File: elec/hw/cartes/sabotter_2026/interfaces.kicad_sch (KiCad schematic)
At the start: 49 parts, among them J10 2-1445051-3, J11 22272051, J12 22272031, J13 3-794630-6, J6 3-794630-4, J9 3-794630-4, U6 TCAN1042DRQ1, U7 TCA6408ARGTR, U8 SN74LVC1T45DBV

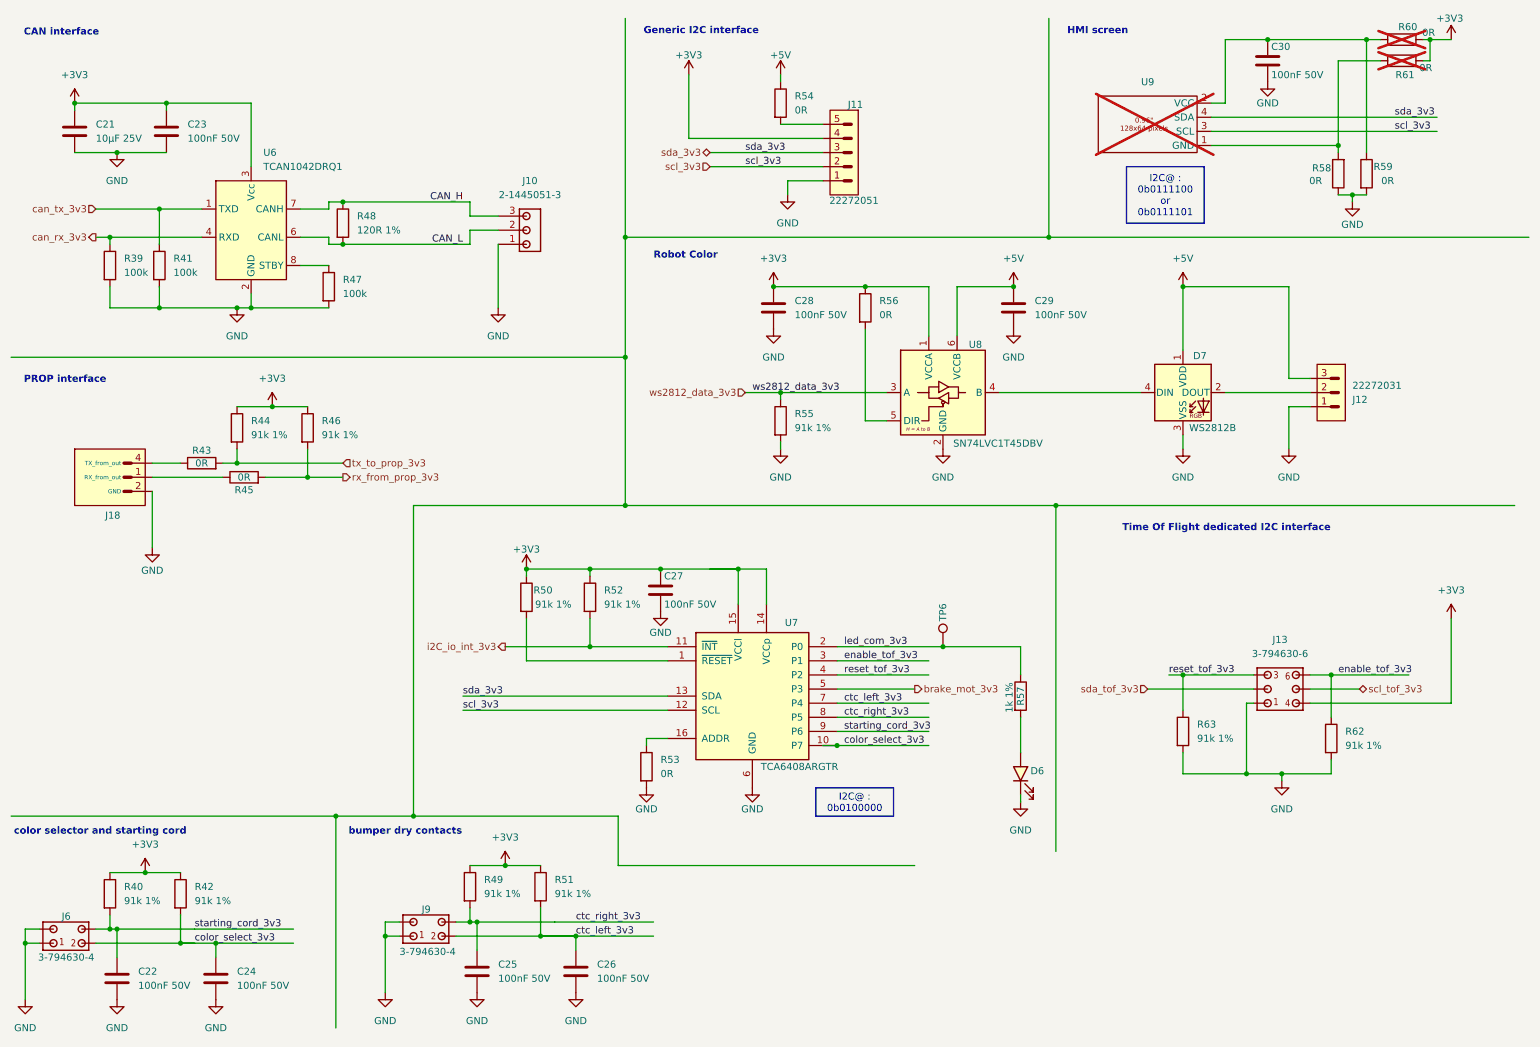
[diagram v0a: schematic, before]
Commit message: sabotter corrections wip
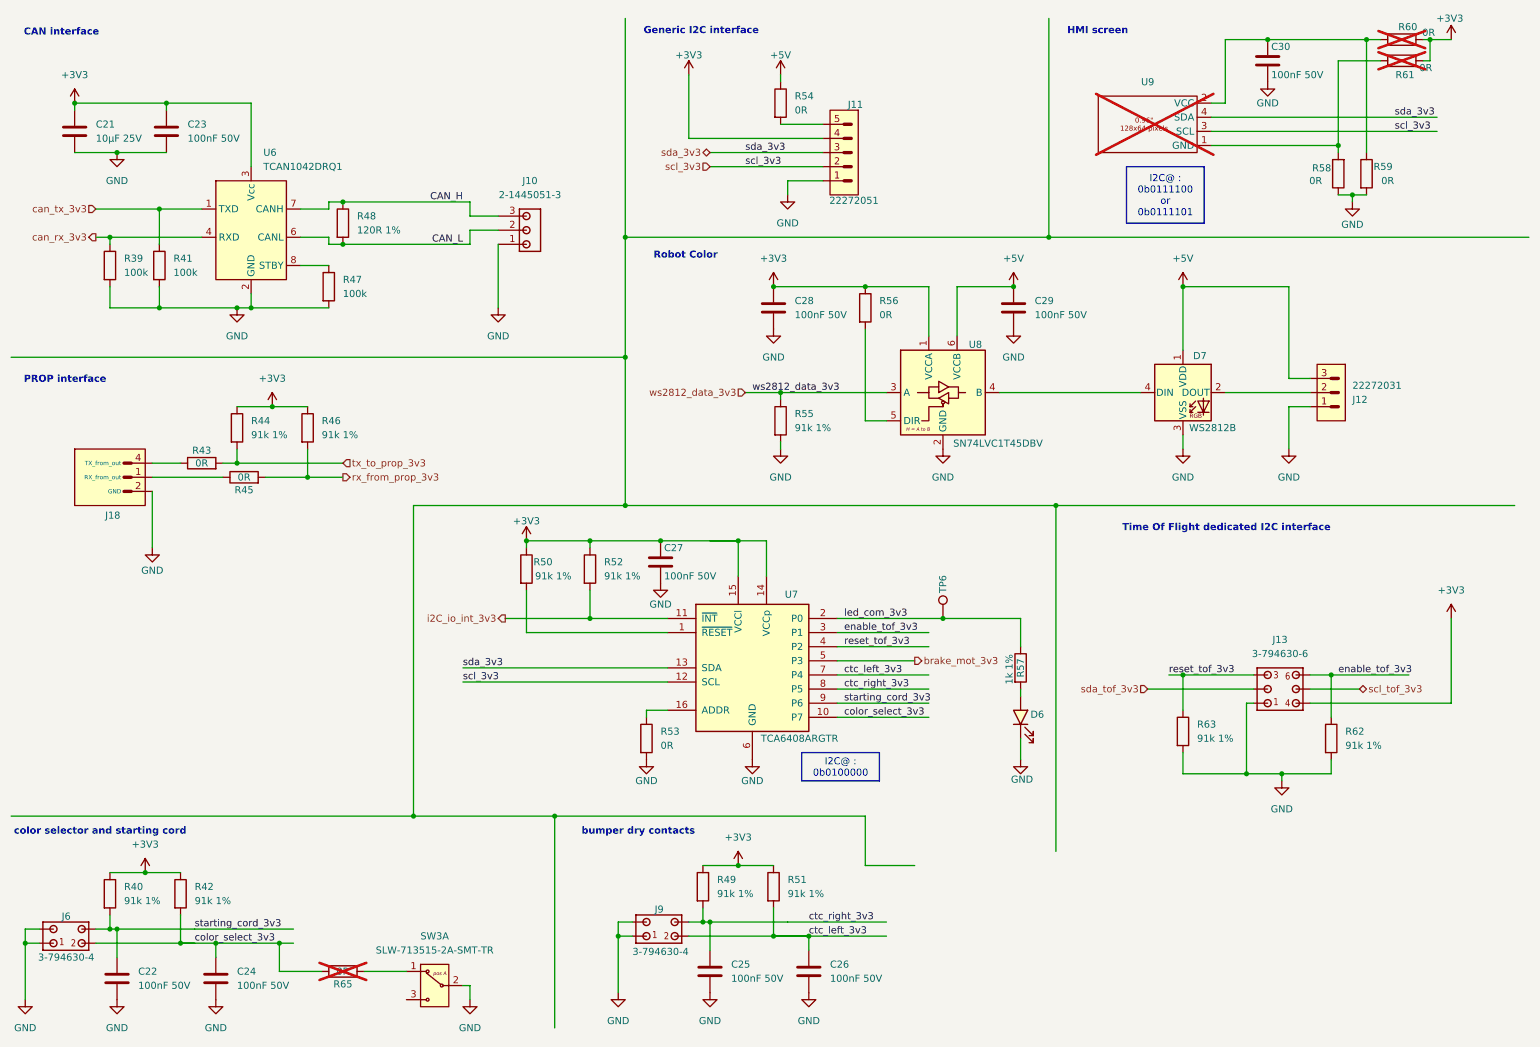
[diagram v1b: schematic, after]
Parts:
- added R65: 0R, cocotter_resistor:r0603_reflow, symbol cocotter_resistors:R_0R_0603
- added SW3: SLW-713515-2A-SMT-TR, cocotter_others:SLW-713515-2A-SMT-TR, symbol cocotter_connectors:SLW-713515-2A-SMT-TR
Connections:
- net GND: now also SW3.2
- net color_select_3v3: now also R65.2
- new net: R65.1, SW3.1
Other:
- moved on the sheet: C25, C26, C27, D6, J9, R49, R50, R51, R52, R53, R57, TP6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
